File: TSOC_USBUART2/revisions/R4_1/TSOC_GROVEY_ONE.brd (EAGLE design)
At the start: 44.5 x 30.5 mm, 43 parts, among them J1 JMP-3-1_2, J2 JMP-3-1_2, U1 CY7C65215-32-PROTO, U2 AP2112K-3.3V

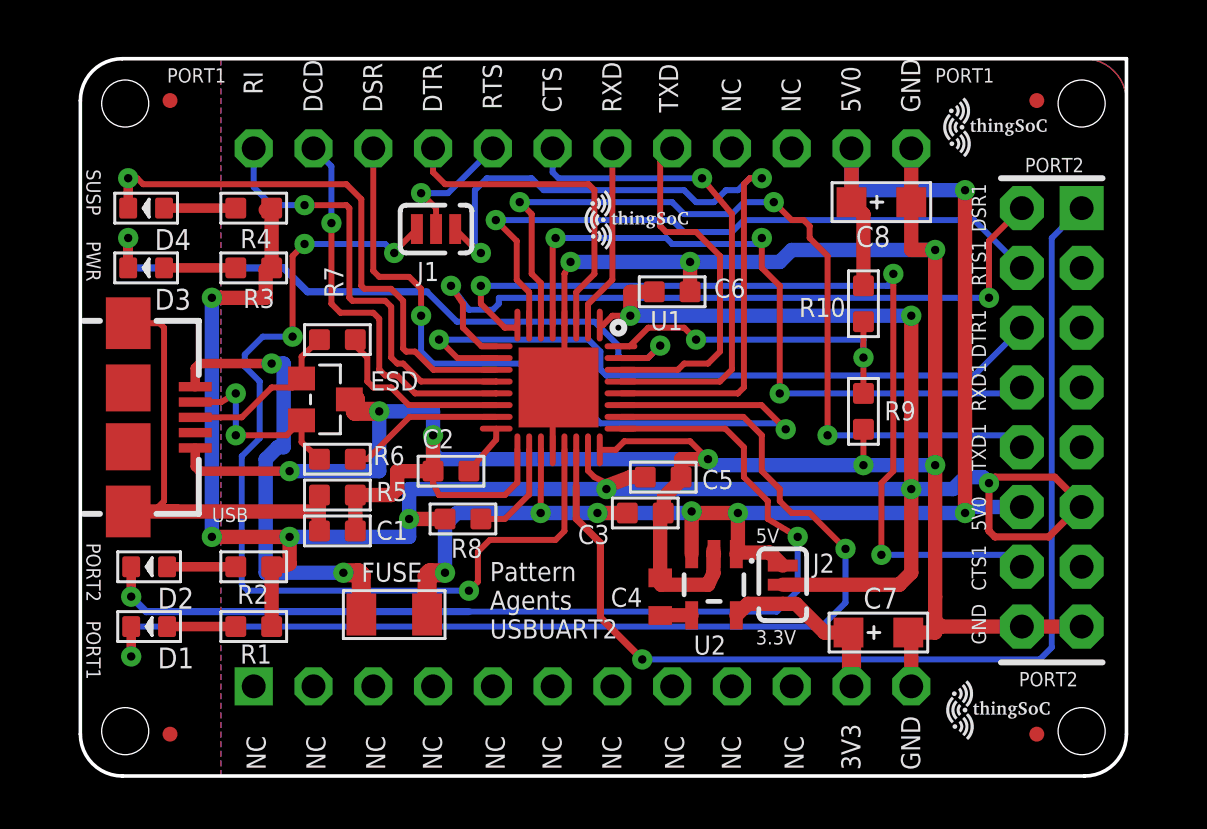
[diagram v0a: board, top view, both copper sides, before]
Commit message: update R5
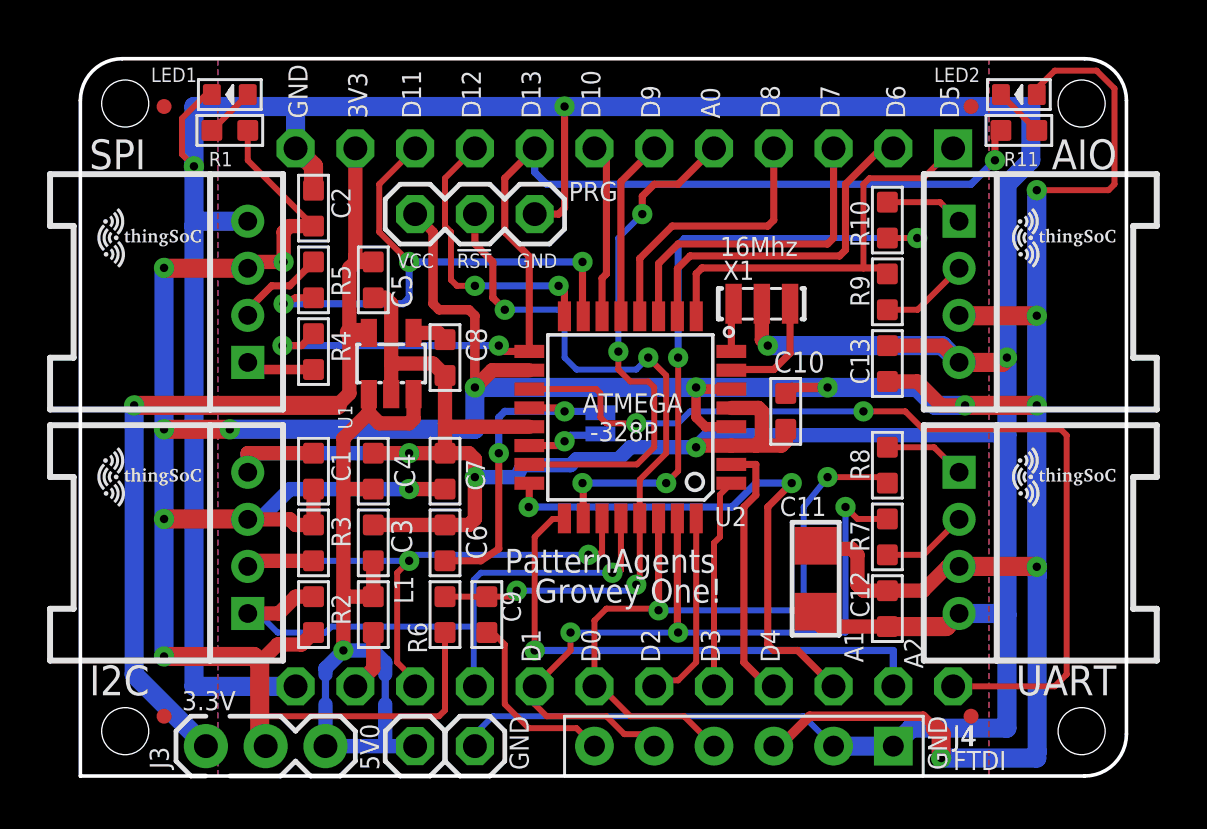
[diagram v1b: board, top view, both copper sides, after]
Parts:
- removed D1: YELLOW-0603, Seeed-LED-2016:LED-0603
- removed D2: BLUE-0603, Seeed-LED-2016:LED-0603
- removed D3: GREEN-0603, Seeed-LED-2016:LED-0603
- removed D4: RED-0603, Seeed-LED-2016:LED-0603
- removed ESD: 5V-225MW, Seeed-Diode-2016:SOT-23
- removed FUSE: SMD1206R500SF, Seeed-Fuse-2016:F1206
- removed J1, J2: JMP-3-1_2, PatternAgents-ProtoPads:JMP-3-1_2
- removed PORT2: (no value), PatternAgents-ProtoPads:2X8
- removed U$4: TSOC-PCB-SINGLE, thingSoC:TSOC-BB-BRD-DIM
- removed U$5, U$6, U$7: TSOC-LOGO-SMALL, thingSoC:TSOC-LOGO-SML
- removed USB: USB_AB, BeeSafe:USB-AB-MICRO-SMD
- added $$U$1: TSOC-PCB-SINGLE, thingSoC:TSOC-BB-BRD-DIM
- added $$U$3, U$101, U$103: TSOC-LOGO-SMALL, thingSoC:TSOC-LOGO-SML
- added 5V0, GND: (no value), PatternAgents-ProtoPads:1X01
- added A7: (no value), PatternAgents-ProtoPads:JMP-2-NO
- added AIO, I2C, SPI, UART: 4P-2.0-90D, Seeed-Connector -2016:HW4-2.0-90D
- added C10, C12, C13, C9: 100nf, Seeed-Capacitor-2016:C0603
- added C11: 22uF, TSOC_USBUART2:EIA-1206
- added J3: NO, PatternAgents-ProtoPads:JMP-3-NO-PTH-2.54
- added J4: 6p-2.54, Seeed-Connector -2016:H6-2.54
- added L1: 120OHM-500MA, Seeed-Inductor-2016:L0603
- added LED1: GREEN-0603, Seeed-LED-2016:LED-0603
- added LED2: RED-0603, Seeed-LED-2016:LED-0603
- added PRG: (no value), PatternAgents-ProtoPads:1X03
- added R11: 1K 1/10W, Seeed-Resistor-2016:R0603
- added U$102: TSOC-LOGO-LRG, thingSoC:TSOC-LOGO-LRG
- added X1: 16MHZ, Seeed-Crystal Oscillator-2016:X3-SMD-3.6X1.3X0.8MM
- $$U$2, U$1, U$3: value TSOC-LOGO -> TSOC-LOGO-SMALL; device thingSoC:TSOC-LOGO-BLANK -> thingSoC:TSOC-LOGO-SML
- C1: value 100pf -> 100nf
- C2: value 1uf -> 100nf
- C3, C5: value 100nf -> 10uf
- C4: value DNP -> 100nf; device TSOC_USBUART2:EIA-0603 -> Seeed-Capacitor-2016:C0603
- C7: value 22uf -> 100nf; device Seeed-Capacitor-2016:AVX-A -> Seeed-Capacitor-2016:C0603
- C8: value 22uf -> 470Pf; device Seeed-Capacitor-2016:AVX-A -> Seeed-Capacitor-2016:C0603
- R1, R4: value 1K -> 1K 1/10W
- R10: value 22K -> 1K 1/10W
- R2, R3: value 1K -> 2.2K
- R5: value 1M -> 1K 1/10W
- R6: value 22R -> 10K 1/10W
- R7: value 22R -> 1K 1/10W
- R8, R9: value 10K -> 1K 1/10W
- U$100: value TSOC-LOGO-LRG -> TSOC-LOGO-SMALL; device thingSoC:TSOC-LOGO-LRG -> thingSoC:TSOC-LOGO-SML
- U1: value CY7C65215-32-PROTO -> XC6204B332MR-SOT23-5; device PatternAgents-Cypress:QFN32-PROTO -> Seeed-IC-2016:SOT-23-5
- U2: value AP2112K-3.3V -> ATMEGA328; device SparkFun-PowerIC:SOT23-5 -> SparkFun:TQFP32-08
- moved $$U$2 38.2 mm to (40.4, 12.7)
- moved U$100 27.7 mm to (4.32, 15.2)
- moved FID3 26.8 mm to (37.8, 28.4)
- moved FID4 26.3 mm to (37.8, 2.54)
- moved R7 24.8 mm to (34.3, 10.2), turned to 0 degrees
- moved U$3 21.2 mm to (1.52, 22.9)
- moved R1 21.1 mm to (6.35, 27.4)
- moved C8 19.7 mm to (15.5, 17.8)
- moved C7 19.7 mm to (15.5, 13.0)
- moved R8 18.2 mm to (34.3, 13.2), turned to 180 degrees
- moved C5 14.9 mm to (12.4, 21.1), turned to 180 degrees
- moved C6 14.4 mm to (15.5, 9.91), turned to 0 degrees
- moved C4 13.3 mm to (12.4, 13.0), turned to 180 degrees
- moved C2 12.6 mm to (9.91, 24.1), turned to 180 degrees
- moved R3 12.0 mm to (9.91, 9.91), turned to 180 degrees
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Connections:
- removed net !CTS: TSOC.6C, U1.29
- removed net !CTS1: PORT2.14, U1.8
- removed net !DCD: TSOC.2C, U1.13
- removed net !DSR: TSOC.3C, U1.27
- removed net !DSR1: PORT2.2, U1.9
- removed net !DTR: TSOC.4C, U1.3
- removed net !DTR1: PORT2.6, U1.10
- removed net !POWER: D3.-, U1.31
- removed net !RI: TSOC.1C, U1.12
- removed net !RTS: J1.1, U1.28
- removed net !RTS1: PORT2.4, U1.7
- removed net !RX_LED: D1.-, U1.26
- removed net !TX_LED: D2.-, U1.25
- removed net !USB_RST: R8.2, U1.18
- removed net BLU: D2.+, R2.1
- removed net BUS_DET: R10.2, R9.1, U1.32
- removed net GRN: D3.+, R3.1
- removed net N$1: J1.2, TSOC.5C
- removed net RED: D4.+, R4.1
- removed net RXD: TSOC.7C, U1.2
- removed net RXD1: PORT2.8, U1.5
- removed net SUSP: D4.-, U1.11
- removed net TXD: TSOC.8C, U1.30
- removed net TXD1: PORT2.10, U1.6
- removed net TXDEN_0: J1.3, U1.21
- removed net TXDEN_1: PORT2.1, U1.22
- removed net USB1_DM: ESD.2, R6.1, USB.D-
- removed net USB1_DP: ESD.1, R7.1, USB.D+
- removed net USB1_ID: USB.ID
- removed net USB1_M: R6.2, U1.15
- removed net USB1_P: R7.2, U1.14
- removed net USB1_SHIELD: C1.1, R5.1, USB.SHIELD1, USB.SHIELD2
- removed net USB1_VBUS: FUSE.1, USB.VBUS
- removed net VCCD1: C2.2, U1.16
- removed net YEL: D1.+, R1.1
- new net !JRST: C9.1, J4.6
- new net !RST: C9.2, PRG.2, R6.1, U2.29
- new net A0: TSOC.5B, U2.23
- new net A1: TSOC.3C, U2.24
- new net A2: TSOC.2C, U2.25
- new net A3: R10.1, U2.26
- new net A3E: AIO.1, R10.2
- new net A4: I2C.2, R3.1, TSOC.10C, U2.27
- new net A5: I2C.1, R2.1, TSOC.9C, U2.28
- new net A6: TSOC.1C, U2.19
- new net A7: A7.1, U2.22
- new net AREF: A7.2, C6.2, U2.20
- new net D0: J4.4, R8.1, TSOC.7C, U2.30
- new net D0E: R8.2, UART.1
- new net D1: J4.5, R7.1, TSOC.8C, U2.31
- new net D10: TSOC.7B, U2.14
- new net D11: R5.2, TSOC.10B, U2.15
- new net D11E: R5.1, SPI.2
- new net D12: TSOC.9B, U2.16
- new net D13: R11.2, R4.2, TSOC.8B, U2.17
- new net D13E: R4.1, SPI.1
- new net D1E: R7.2, UART.2
- new net D2: TSOC.6C, U2.32
- new net D3: TSOC.5C, U2.1
- new net D4: TSOC.4C, U2.2
- new net D5: R9.1, TSOC.1B, U2.9
- new net D5E: AIO.2, R9.2
- new net D6: TSOC.2B, U2.10
- new net D7: TSOC.3B, U2.11
- new net D8: TSOC.4B, U2.12
- new net D9: TSOC.6B, U2.13
- new net LEDR: LED2.-, R11.1
- new net N$17: LED1.+, R1.1
- new net TSOC_5V0: L1.2, TSOC.11C
- new net XIN: U2.7, X1.3
- new net XOUT: U2.8, X1.1
- net 3V3: now also C5.2, J3.1, U1.5; no longer C7.+, J2.1, U2.5
- net 5V0: now also 5V0.1, C3.2, C4.1, J3.3, L1.1, U1.1, U1.3; no longer C3.1, C8.+, FUSE.2, J2.3, PORT2.12, R10.1, TSOC.11C, U1.19, U2.1, U2.3
- net BYPASS1: now also C8.1, U1.4; no longer C4.1, U2.4
- net GND: now also AIO.4, C10.1, C11.2, C12.2, C13.2, C2.2, C3.1, C7.1, C8.2, GND.1, I2C.4, J4.1, J4.2, LED1.-, PRG.3, SPI.4, U1.2, U2.21, U2.3, U2.5, UART.4, X1.2; no longer C2.1, C3.2, C7.-, C8.-, ESD.3, PORT2.15, PORT2.16, R5.2, R9.2, U1.17, U1.20, U1.24, U1.4, U1.EXP, U2.2, USB.GND
- net VCC: now also AIO.3, C1.1, C10.2, C11.1, C12.1, C13.1, C2.1, C7.2, I2C.3, J3.2, J4.3, LED2.+, PRG.1, R6.2, SPI.3, U2.18, U2.4, U2.6, UART.3; no longer C5.2, C6.2, J2.2, PORT2.11, R4.2, R8.1, U1.1, U1.23
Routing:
- net GND: track 125.9 -> 226.8 mm, vias 9 -> 7
- net VCC: track 105.1 -> 194.2 mm, vias 9 -> 16
- net !RX_LED: track 48.8 -> 0.00 mm, vias 2 -> 0
- net TXDEN_1: track 46.9 -> 0.00 mm, vias 1 -> 0
- net D13: track 0.00 -> 44.3 mm, vias 0 -> 3
- net !TX_LED: track 43.0 -> 0.00 mm, vias 2 -> 0
- net TXDEN_0: track 41.3 -> 0.00 mm, vias 4 -> 0
- net A6: track 0.00 -> 39.9 mm, vias 0 -> 2
- net !CTS1: track 39.2 -> 0.00 mm, vias 3 -> 0
- net TXD1: track 36.4 -> 0.00 mm, vias 3 -> 0
- net !DSR: track 35.6 -> 0.00 mm, vias 2 -> 0
- net D1: track 0.00 -> 33.4 mm, vias 0 -> 3
- net 5V0: track 65.6 -> 32.4 mm, vias 7 -> 1
- net !RTS: track 32.4 -> 0.00 mm, vias 2 -> 0
- net !RST: track 0.00 -> 31.8 mm, vias 0 -> 4
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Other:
- outline, holes or cut-outs redrawn
- board text added: "!CTS"
- board text added: "!DTR"
- board text added: "!RST"
- board text added: "16Mhz"
- board text added: "A0"
- board text added: "A1"
- board text added: "A2"
- board text added: "A3"
- board text added: "A4"
- board text added: "A5"
- board text added: "A6"
- board text added: "AIO"
- board text added: "ATMEGA -328P"
- board text added: "D0"
- board text added: "D1"
- board text added: "D10"
- board text added: "D11"
- board text added: "D12"
- board text added: "D13"
- board text added: "D2"
- board text added: "D3"
- board text added: "D4"
- board text added: "D5"
- board text added: "D6"
- board text added: "D7"
- board text added: "D8"
- board text added: "D9"
- board text added: "FTDI"
- board text added: "Grovey One!"
- board text added: "I2C"
- board text added: "J3"
- board text added: "J4"
- board text added: "Rev. 2.0"
- board text added: "SPI"
- board text added: "TSOC_GROVEY_ONE!"
- board text added: "UART"
- board text removed: "5V"
- board text removed: "CTS"
- board text removed: "CTS1"
- board text removed: "DCD"
- board text removed: "DSR"
- board text removed: "DSR1"
- board text removed: "DTR"
- board text removed: "DTR1"
- board text removed: "NC"
- board text removed: "PORT1"
- board text removed: "PORT2"
- board text removed: "PWR"
- board text removed: "Pattern Agents USBUART2"
- board text removed: "RI"
- board text removed: "RTS"
- board text removed: "RTS1"
- board text removed: "RXD"
- board text removed: "RXD1"
- board text removed: "Rev. 5.1"
- board text removed: "SUSP"
- board text removed: "TSOC_USBUART2"
- board text removed: "TXD"
- board text removed: "TXD1"
